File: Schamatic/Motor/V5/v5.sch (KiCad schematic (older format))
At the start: 47 parts, among them J1 SWD, J10 GND, J11 V, J12 U, J13 W, J2 SPI, J3 RS485, J4 RS485, J5 CAP+, J6 12, J7 12, J8 CAP-, J9 GND, Q1 PSMN3R3-40YS, Q2 PSMN3R3-40YS, Q3 PSMN3R3-40YS, Q4 PSMN3R3-40YS, Q5 PSMN3R3-40YS, Q6 PSMN3R3-40YS, SW1 SWiTCH, SW2 SWiTCH, U1 STSPIN32F0, U2 LTC2876, Y1 8Mhz

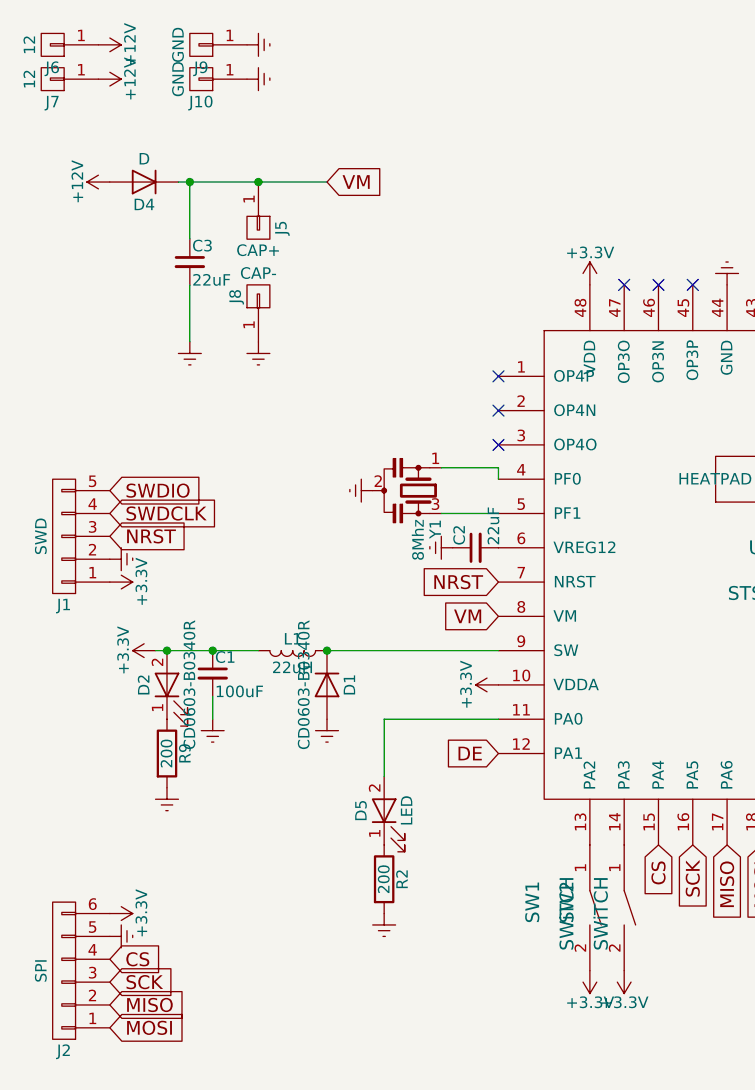
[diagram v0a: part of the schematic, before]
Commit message: new version of the board
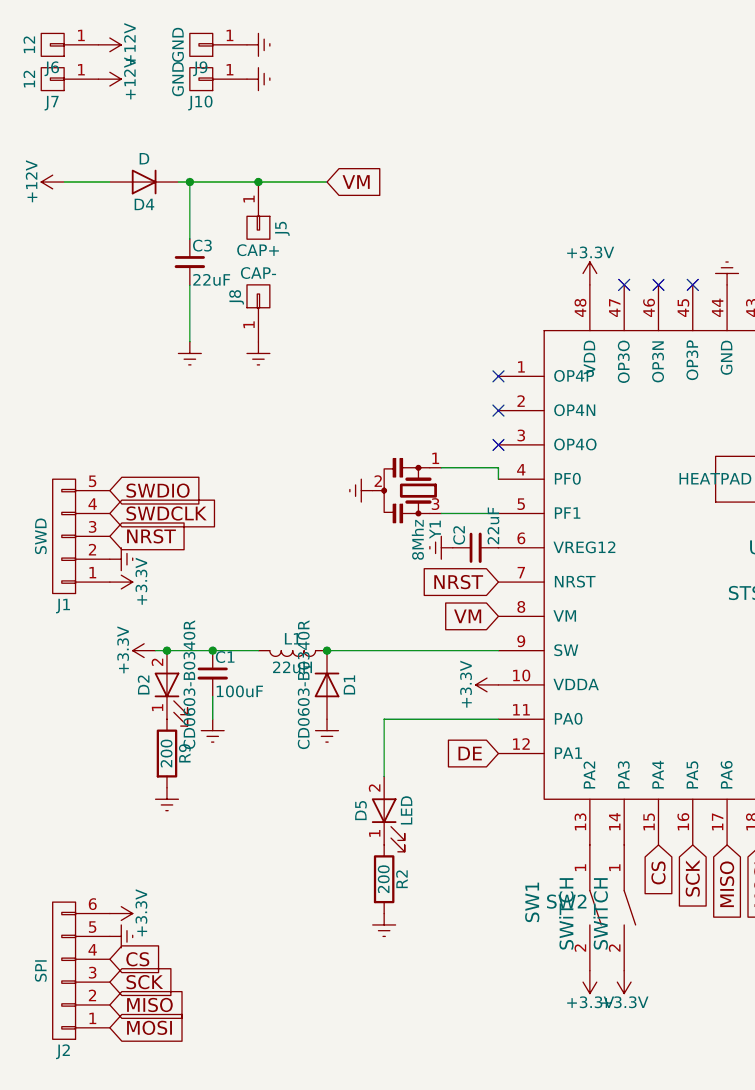
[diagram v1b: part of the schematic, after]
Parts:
- D1: footprint Diodes_SMD:D_0805 -> Diodes_SMD:D_0603
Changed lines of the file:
@@
 F 0 "D1" H 1900 3600 50  0000 C CNN
 F 1 "CD0603-B0340R" H 1900 3400 50  0000 C CNN
-F 2 "Diodes_SMD:D_0805" H 1900 3500 50  0001 C CNN
+F 2 "Diodes_SMD:D_0603" H 1900 3500 50  0001 C CNN
 F 3 "" H 1900 3500 50  0001 C CNN
 	1    1900 3500
@@
 L +12V #PWR06
 U 1 1 597768BB
-P 950 1300
-F 0 "#PWR06" H 950 1150 50  0001 C CNN
-F 1 "+12V" H 950 1440 50  0000 C CNN
-F 2 "" H 950 1300 50  0001 C CNN
-F 3 "" H 950 1300 50  0001 C CNN
-	1    950  1300
+P 750 1300
+F 0 "#PWR06" H 750 1150 50  0001 C CNN
+F 1 "+12V" H 750 1440 50  0000 C CNN
+F 2 "" H 750 1300 50  0001 C CNN
+F 3 "" H 750 1300 50  0001 C CNN
+	1    750  1300
 	0    -1   -1   0
 $EndComp
@@
 U 1 1 59C795D7
 P 2650 4500
-F 0 "SW2" H 2600 4800 60  0000 C CNN
+F 0 "SW2" V 2600 4800 60  0000 C CNN
 F 1 "SWiTCH" H 2650 4950 60  0000 C CNN
 F 2 "Resistors_SMD:R_1206" H 2650 4500 60  0001 C CNN
@@
 	1    0    0    -1
 $EndComp
+Wire Wire Line
+	950  1300 750  1300
 $EndSCHEMATC
